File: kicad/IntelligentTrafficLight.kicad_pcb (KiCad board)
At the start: 4 copper layers, 100 x 140 mm, 124 parts, among them J1 Conn_01x03_Pin, J2 Conn_01x10_Socket, J3 USB-C Receptacle, J4 Conn_01x07_Socket, J5 Conn_01x07_Socket, SW1 Pushbutton, SW2 Pushbutton, U1 ESP32-C3-MINI-1-H4X, U2 PCA9685PW, U3 TLV76133DCY, U4 MAX40200AUK, U5 TLC555xD, U6 TLC555xD, U7 TLC555xD

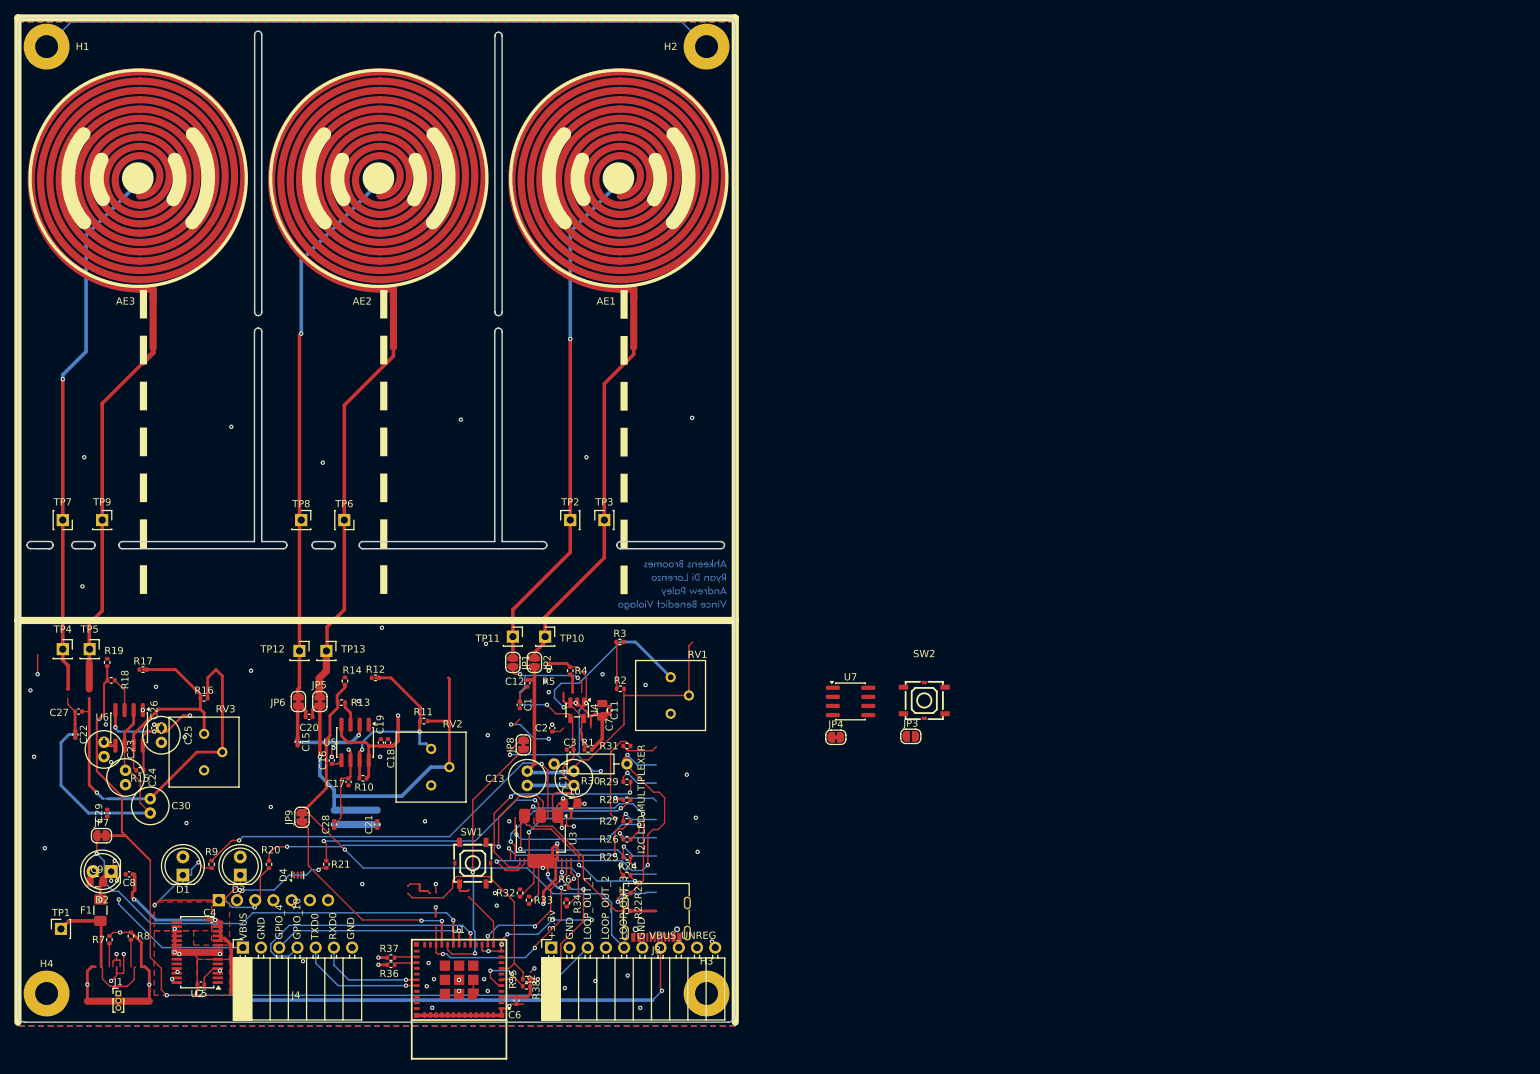
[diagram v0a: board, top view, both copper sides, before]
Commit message: update!
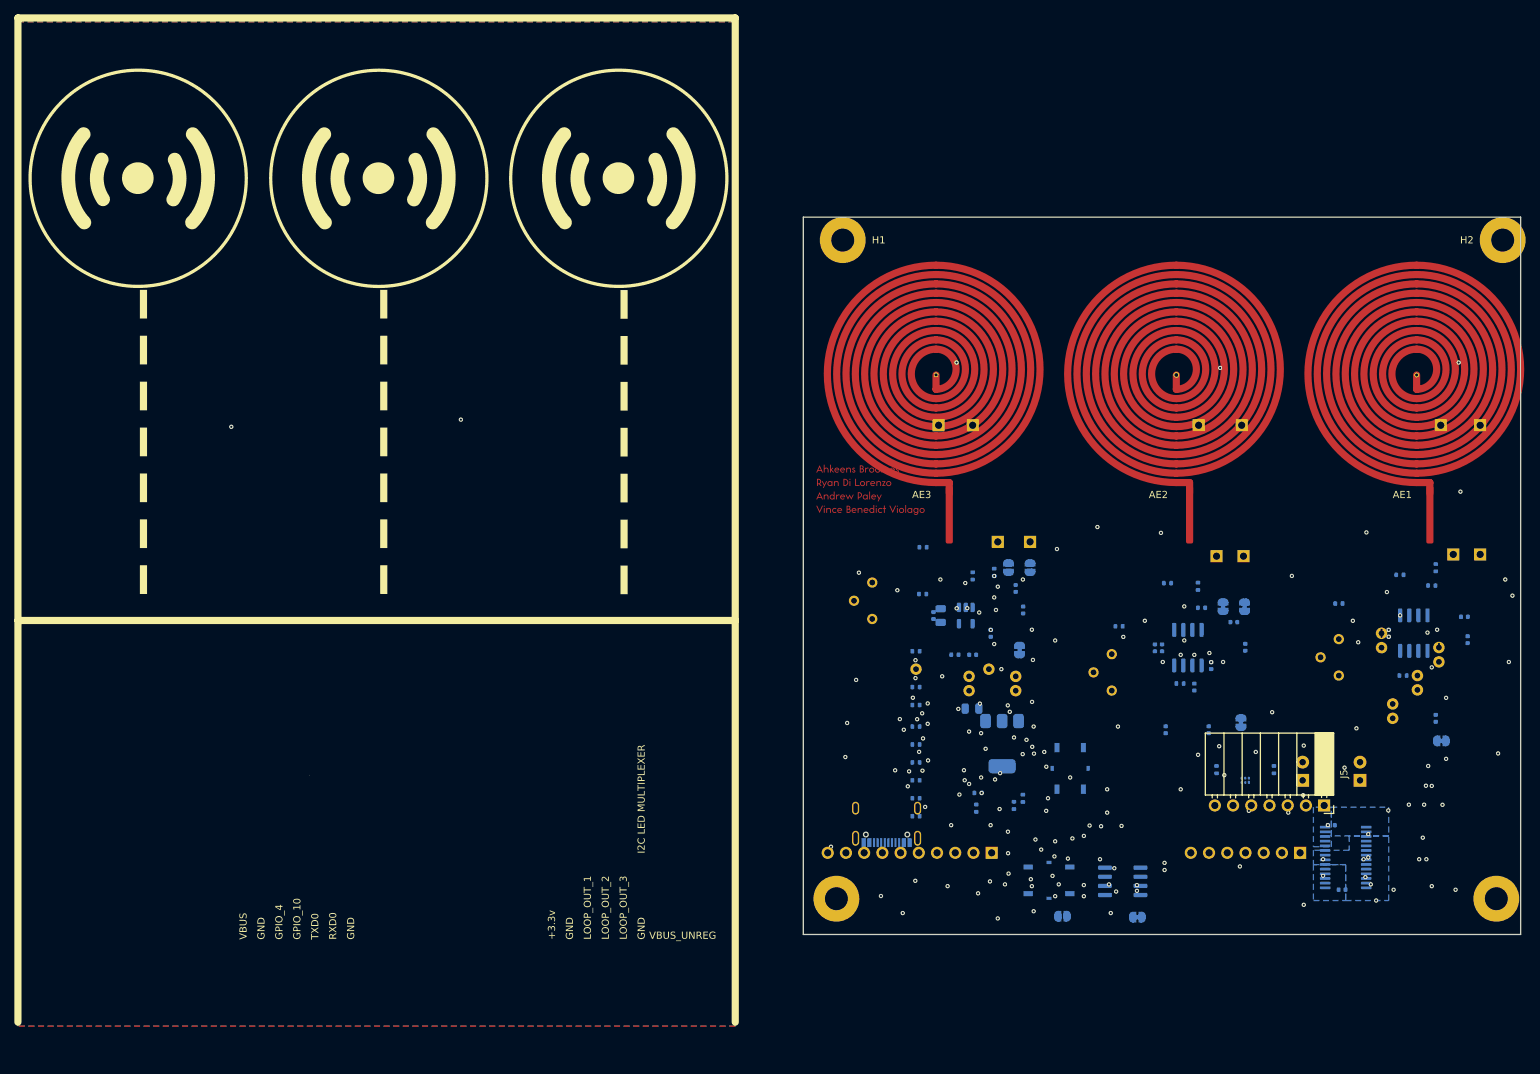
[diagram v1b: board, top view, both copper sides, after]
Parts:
- removed C6: 100nF, Capacitor_SMD:C_0402_1005Metric
- removed C8: 10uF, Capacitor_SMD:C_0402_1005Metric
- removed C9: 22uF, Capacitor_SMD:C_0805_2012Metric
- removed D2: LED, LED_THT:LED_D5.0mm
- removed F1: 1.5A, Fuse:Fuse_1206_3216Metric_Pad1.42x1.75mm_HandSolder
- removed J1: Conn_01x03_Pin, Connector_PinHeader_1.00mm:PinHeader_1x03_P1.00mm_Vertical
- removed R35, R7, R8: 0, Resistor_SMD:R_0402_1005Metric
- removed R36: 5k, Resistor_SMD:R_0402_1005Metric
- removed R37: 1k, Resistor_SMD:R_0402_1005Metric
- removed R38: 1.5k, Resistor_SMD:R_0402_1005Metric
- removed TP1: VBUS, Connector_PinSocket_2.54mm:PinSocket_1x01_P2.54mm_Vertical
- removed U1: ESP32-C3-MINI-1-H4X, EASYEDA2KICAD:WIFIM-SMD_ESP32-C3-MINI-1
- C1, C10, C11, C12, C13, C14, C15, C16, C17, C18, C19, C2, C20, C21, C22, C23, C24, C25, C26, C27, C28, C29, C3, C30, C4, C5, C7, D1, D3, D4, H3, H4, J2, J3, J4, JP1, JP2, JP3, JP4, JP5, JP6, JP7, JP8, JP9, R1, R10, R11, R12, R13, R14, R15, R16, R17, R18, R19, R2, R20, R21, R22, R23, R24, R25, R26, R27, R28, R29, R3, R30, R31, R32, R33, R34, R4, R5, R6, R9, RV1, RV2, RV3, SW1, SW2, TP10, TP11, TP12, TP13, TP2, TP3, TP4, TP5, TP6, TP7, TP8, TP9, U2, U3, U4, U5, U6, U7: moved to B.Cu
- J5, kibuzzard-691CE1C1: moved to F.Cu
- moved H4 202.5 mm to (270.1, 142.8), turned to 180 degrees
- moved TP4 198.0 mm to (267.8, 94.8), turned to 180 degrees
- moved TP7 198.0 mm to (267.8, 76.8)
- moved C22 194.5 mm to (266.1, 106.7)
- moved C27 193.7 mm to (265.7, 103.5), turned to 180 degrees
- moved TP5 190.6 mm to (264.1, 94.8), turned to 180 degrees
- moved JP7 187.3 mm to (262.4, 120.8), turned to 180 degrees
- moved TP9 187.1 mm to (262.3, 76.8), turned to 180 degrees
- moved C23 186.6 mm to (262.1, 107.8)
- moved C29 185.7 mm to (261.7, 117.6)
- moved R19 185.7 mm to (261.7, 96.6)
- moved R18 184.6 mm to (261.1, 99.1), turned to 0 degrees
- moved C24 180.6 mm to (259.1, 111.7)
- moved U6 179.6 mm to (258.6, 105.8)
- moved R15 176.6 mm to (257.1, 111.7), turned to 0 degrees
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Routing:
- net (no net): track 441.3 -> 0.00 mm
- net GND: track 366.9 -> 0.00 mm, vias 83 -> 81
- net +5V: track 199.1 -> 0.00 mm, vias 12 -> 10
- net /GPIO_5: track 135.4 -> 0.00 mm
- net /LOOP_OUT_1: track 126.9 -> 0.00 mm
- net +3.3V: track 117.6 -> 0.00 mm, vias 14 -> 16
- net VBUS_{unregulated}: track 94.8 -> 0.00 mm, vias 4 -> 3
- net Net-(JP6-A): track 76.6 -> 0.00 mm
- net /Inductive Loop/OUT3: track 76.4 -> 0.00 mm, vias 3 -> 4
- net /LOOP_OUT_3: track 75.7 -> 0.00 mm
- net /LOOP_OUT_2: track 70.3 -> 0.00 mm, vias 3 -> 2
- net Net-(U2-LED0): track 59.6 -> 0.00 mm
- net Net-(U5-DIS): track 57.6 -> 0.00 mm
- net Net-(JP5-B): track 56.9 -> 0.00 mm
- net Net-(JP5-A): track 56.7 -> 0.00 mm
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- added copper zone on B.Cu, net +3.3V
- added copper zone on In2.Cu, net +3.3V
- added copper zone on B.Cu, net VBUS_{unregulated}
- removed copper zone on F.Cu, net +3.3V
- removed copper zone on F.Cu, net VBUS_{unregulated}
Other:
- board size 100 x 140 mm -> 100 x 100 mm
